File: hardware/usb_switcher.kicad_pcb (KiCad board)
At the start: 2 copper layers, 21 x 52.5 mm, 20 parts, among them U1 MCP1700, U2 IM41_3VDC, U3 IM41_3VDC

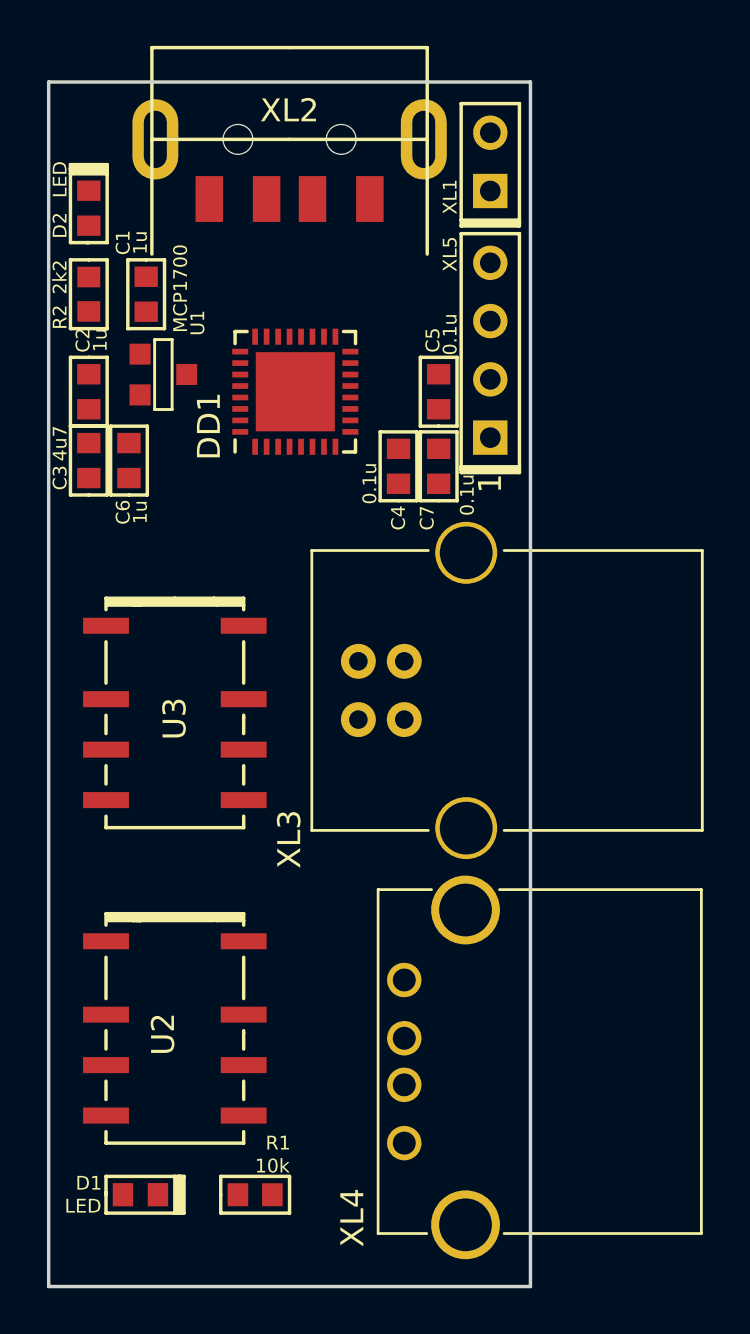
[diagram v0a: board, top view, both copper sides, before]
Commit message: Complete PCB
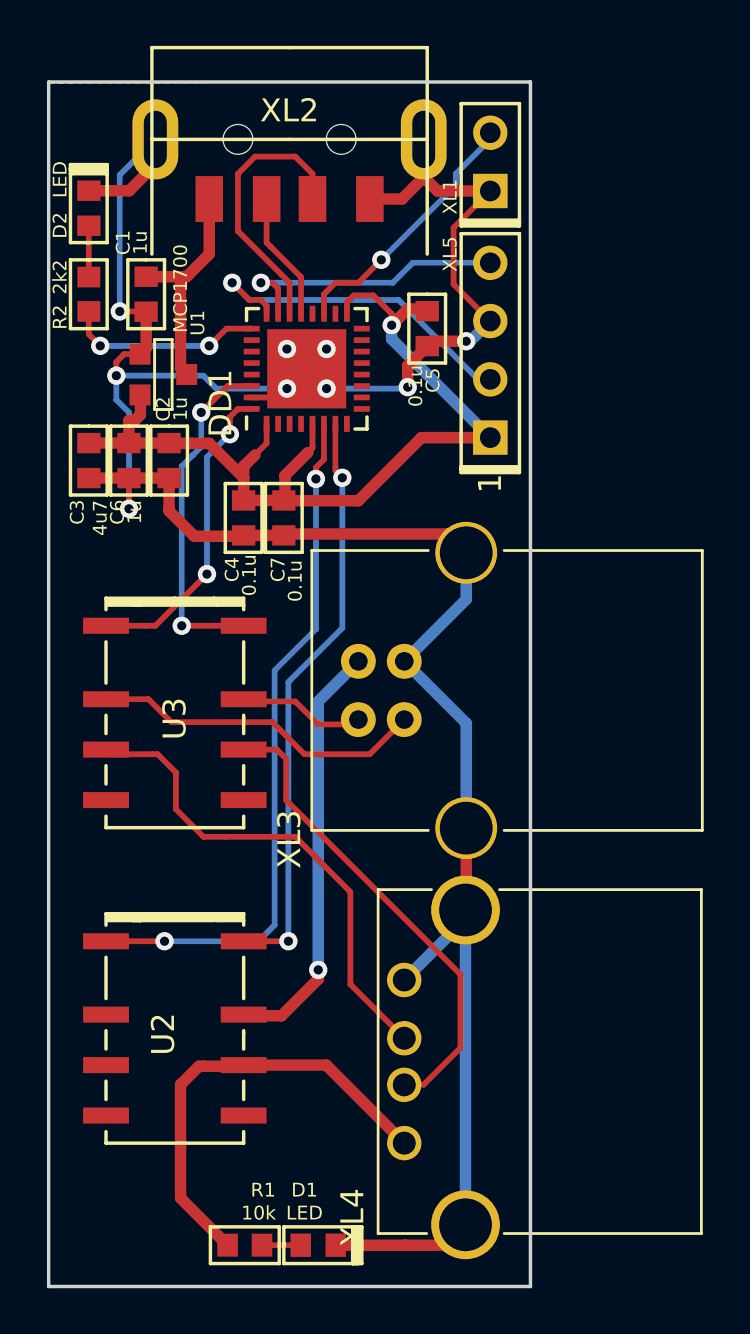
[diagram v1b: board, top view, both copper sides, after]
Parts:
- moved D1 8.06 mm to (181.0, 103.2)
- moved C4 7.12 mm to (177.8, 71.5), turned to 270 degrees
- moved C7 7.12 mm to (179.5, 71.5), turned to 270 degrees
- moved C2 4.61 mm to (174.5, 69.0)
- moved C5 2.80 mm to (185.8, 63.2), turned to 270 degrees
- moved R1 2.25 mm to (177.8, 103.2), turned to 180 degrees
- moved DD1 1.12 mm to (180.5, 65.0)
- turned C3 to 270 degrees
- turned C6 to 270 degrees
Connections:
- DD1 pad 10: /POWER_LED -> Net-(DD1-Pad10)
- DD1 pad 25: Net-(DD1-Pad25) -> /POWER_LED
- DD1 pad 30: Net-(DD1-Pad30) -> /RELAY_DATA_2
- DD1 pad 32: Net-(DD1-Pad32) -> /RELAY_DATA_1
- DD1 pad 8: /RELAY_DATA_1 -> Net-(DD1-Pad8)
- DD1 pad 9: /RELAY_DATA_2 -> Net-(DD1-Pad9)
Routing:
- net GND: track 0.00 -> 125.7 mm, vias 0 -> 9
- net +3.3V: track 0.00 -> 41.6 mm, vias 0 -> 1
- net /RELAY_POWER_1: track 0.00 -> 30.4 mm, vias 0 -> 2
- net /RELAY_POWER_2: track 0.00 -> 25.6 mm, vias 0 -> 2
- net /DEVICE_DP: track 0.00 -> 21.9 mm
- net /DEVICE_DM: track 0.00 -> 20.9 mm
- net /DEVICE_POWER: track 0.00 -> 19.4 mm
- net /HOST_POWER: track 0.00 -> 18.5 mm, vias 0 -> 1
- net /SWCLK: track 0.00 -> 15.3 mm, vias 0 -> 1
- net /RELAY_DATA_2: track 0.00 -> 15.0 mm, vias 0 -> 2
- net /HOST_DP: track 0.00 -> 14.8 mm
- net /RELAY_DATA_1: track 0.00 -> 13.7 mm, vias 0 -> 2
- net /SWDIO: track 0.00 -> 12.3 mm, vias 0 -> 1
- net /USB_DP: track 0.00 -> 12.0 mm
- net /DBG_TX: track 0.00 -> 11.5 mm, vias 0 -> 1
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- added copper zone on B.Cu, net GND
- added copper zone on F.Cu, net GND
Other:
- net class Default: clearance 0.2 -> 0.1; via_dia 0.6 -> 0.8
- net class PWR added: clearance 0.2, trace_width 0.5, via_dia 0.8, via_drill 0.4
- net class Small PWR added: clearance 0.2, trace_width 0.25, via_dia 0.8, via_drill 0.4
- rule trace_clearance: 0.2 -> 0.1

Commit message: + Fix pcd + Add gerber files
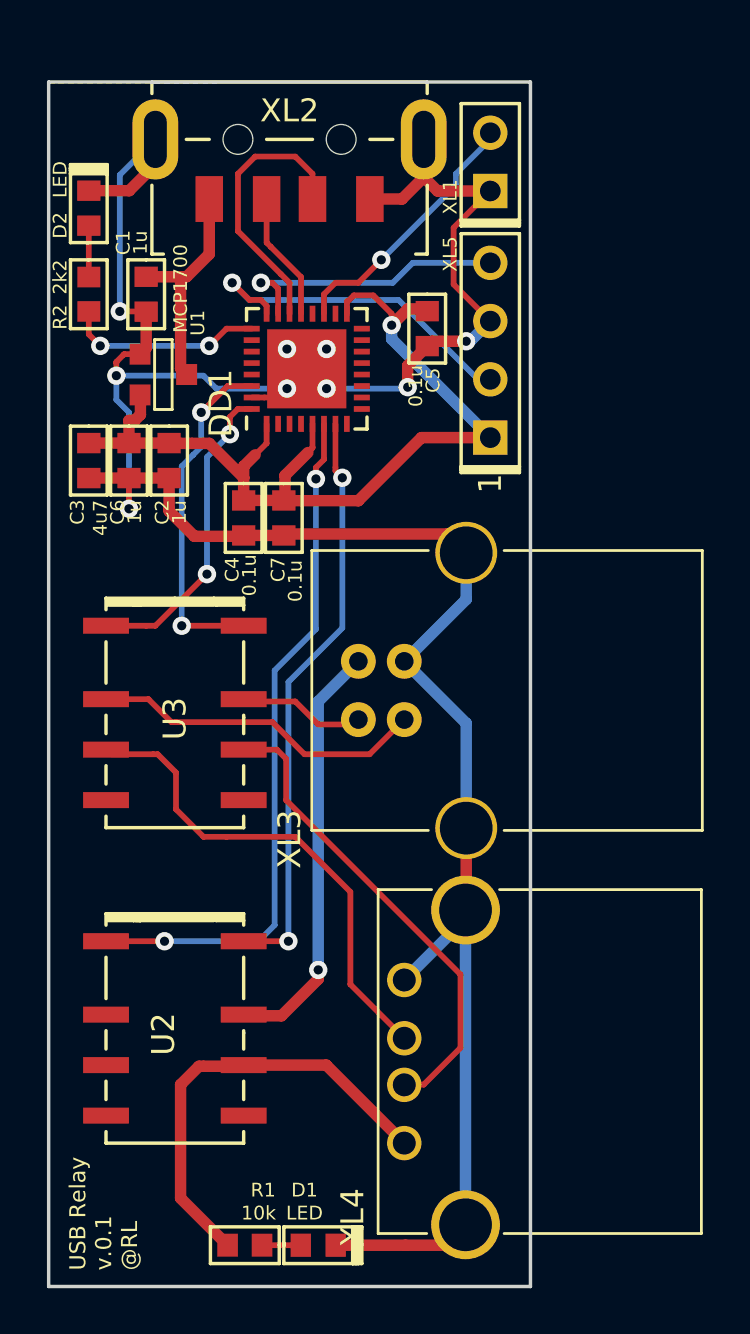
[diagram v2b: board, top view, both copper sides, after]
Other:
- board text added: "USB Relay v.0.1 @RL"
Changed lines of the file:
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@@
     (area 153.000001 47.875 200.725 105.075001)
     (thickness 1.6)
-    (drawings 5)
+    (drawings 6)
     (tracks 265)
     (zones 0)
@@
     (add_net GND)
   )
+  (module Connectors:USB_A_Type2_PCB (layer F.Cu)
+    (at 179.75 55)
+    (descr SHLD)
+    (fp_text reference XL2 (at 0 -1.25) (layer F.SilkS)
+      (effects (font (size 1 1) (thickness 0.15)))
+    )
+    (fp_text value USB_A (at 0 -6) (layer F.Fab)
+      (effects (font (size 1 1) (thickness 0.15)))
+    )
+    (fp_line (start 6 2) (end 6 5) (layer F.SilkS) (width 0.15))
+    (fp_line (start -6 2) (end -6 5) (layer F.SilkS) (width 0.15))
+    (fp_line (start 5.5 5) (end 6 5) (layer F.SilkS) (width 0.15))
+    (fp_line (start -6 5) (end -5.5 5) (layer F.SilkS) (width 0.15))
+    (fp_line (start 3.5 0) (end 4.5 0) (layer F.SilkS) (width 0.15))
+    (fp_line (start -1 0) (end 1 0) (layer F.SilkS) (width 0.15))
+    (fp_line (start -4.5 0) (end -3.5 0) (layer F.SilkS) (width 0.15))
+    (fp_line (start 6 -2.5) (end 6 -2) (layer F.SilkS) (width 0.15))
+    (fp_line (start -6 -2.5) (end -6 -2) (layer F.SilkS) (width 0.15))
+    (fp_line (start -6 -2.5) (end 6 -2.5) (layer F.SilkS) (width 0.15))
+    (pad 1 smd rect (at -3.5 2.6) (size 1.2 2) (layers F.Cu F.Paste F.Mask)
+      (net 1 +5V))
+    (pad 2 smd rect (at -1 2.6) (size 1.2 2) (layers F.Cu F.Paste F.Mask)
+      (net 23 /USB_DM))
+    (pad 3 smd rect (at 1 2.6) (size 1.2 2) (layers F.Cu F.Paste F.Mask)
+      (net 24 /USB_DP))
+    (pad 4 smd rect (at 3.5 2.6) (size 1.2 2) (layers F.Cu F.Paste F.Mask)
+      (net 2 GND))
+    (pad "" np_thru_hole circle (at -2.25 0) (size 1.3 1.3) (drill 1.3) (layers *.Cu *.Mask F.SilkS))
+    (pad "" np_thru_hole circle (at 2.25 0) (size 1.3 1.3) (drill 1.3) (layers *.Cu *.Mask F.SilkS))
+    (pad 5 thru_hole oval (at 5.85 0) (size 2 3.5) (drill oval 1 2.5) (layers *.Cu *.Mask F.SilkS)
+      (net 2 GND))
+    (pad 5 thru_hole oval (at -5.85 0) (size 2 3.5) (drill oval 1 2.5) (layers *.Cu *.Mask F.SilkS)
+      (net 2 GND))
+  )
   (module Capacitors:CAP_0603 (layer F.Cu)
     (at 173.5 61.75 270)
@@
     (at 174.5 69 270)
     (attr smd)
-    (fp_text reference C2 (at -2.25 0.25 450) (layer F.SilkS)
-      (effects (font (size 0.6 0.6) (thickness 0.15)))
-    )
-    (fp_text value 1u (at -2.25 -0.5 270) (layer F.SilkS)
+    (fp_text reference C2 (at 2.25 0.3 450) (layer F.SilkS)
+      (effects (font (size 0.6 0.6) (thickness 0.15)))
+    )
+    (fp_text value 1u (at 2.25 -0.45 270) (layer F.SilkS)
       (effects (font (size 0.6 0.6) (thickness 0.15)))
     )
@@
     )
   )
-  (module Connectors:USB_A_Type2_PCB (layer F.Cu)
-    (at 179.75 55)
-    (descr SHLD)
-    (fp_text reference XL2 (at 0 -1.25) (layer F.SilkS)
-      (effects (font (size 1 1) (thickness 0.15)))
-    )
-    (fp_text value USB_A (at 0 -6) (layer F.Fab)
-      (effects (font (size 1 1) (thickness 0.15)))
-    )
-    (fp_line (start 6 0) (end 6 5) (layer F.SilkS) (width 0.15))
-    (fp_line (start -6 0) (end -6 5) (layer F.SilkS) (width 0.15))
-    (fp_line (start 0 -4) (end 6 -4) (layer F.SilkS) (width 0.15))
-    (fp_line (start 6 -4) (end 6 0) (layer F.SilkS) (width 0.15))
-    (fp_line (start 0 -4) (end -6 -4) (layer F.SilkS) (width 0.15))
-    (fp_line (start -6 -4) (end -6 0) (layer F.SilkS) (width 0.15))
-    (fp_line (start 0 0) (end 6 0) (layer F.SilkS) (width 0.15))
-    (fp_line (start 0 0) (end -6 0) (layer F.SilkS) (width 0.15))
-    (pad 1 smd rect (at -3.5 2.6) (size 1.2 2) (layers F.Cu F.Paste F.Mask)
-      (net 1 +5V))
-    (pad 2 smd rect (at -1 2.6) (size 1.2 2) (layers F.Cu F.Paste F.Mask)
-      (net 23 /USB_DM))
-    (pad 3 smd rect (at 1 2.6) (size 1.2 2) (layers F.Cu F.Paste F.Mask)
-      (net 24 /USB_DP))
-    (pad 4 smd rect (at 3.5 2.6) (size 1.2 2) (layers F.Cu F.Paste F.Mask)
-      (net 2 GND))
-    (pad "" np_thru_hole circle (at -2.25 0) (size 1.3 1.3) (drill 1.3) (layers *.Cu *.Mask F.SilkS))
-    (pad "" np_thru_hole circle (at 2.25 0) (size 1.3 1.3) (drill 1.3) (layers *.Cu *.Mask F.SilkS))
-    (pad 5 thru_hole oval (at 5.85 0) (size 2 3.5) (drill oval 1 2.5) (layers *.Cu *.Mask F.SilkS)
-      (net 2 GND))
-    (pad 5 thru_hole oval (at -5.85 0) (size 2 3.5) (drill oval 1 2.5) (layers *.Cu *.Mask F.SilkS)
-      (net 2 GND))
-  )
   (module Connectors:PLS-4 (layer F.Cu)
     (at 188.5 68 90)
@@
       (net 41 /SWDIO))
   )
+  (gr_text "USB Relay\nv.0.1\n@RL" (at 171.65 104.3 90) (layer F.SilkS)
+    (effects (font (size 0.7 0.7) (thickness 0.175)) (justify left))
+  )
   (gr_line (start 169.25 105) (end 169.25 52.5) (angle 90) (layer Edge.Cuts) (width 0.15))
   (gr_line (start 190.25 105) (end 169.25 105) (angle 90) (layer Edge.Cuts) (width 0.15))
@@
   (segment (start 172.2 66.35) (end 172.75 66.9) (width 0.25) (layer B.Cu) (net 2))
   (segment (start 172.2 65.3) (end 172.2 66.35) (width 0.25) (layer B.Cu) (net 2))
-  (segment (start 172.75 71.1) (end 172.75 69.762) (width 0.25) (layer F.Cu) (net 2) (status 800000))
+  (segment (start 172.75 71.1) (end 172.75 69.762) (width 0.25) (layer F.Cu) (net 2))
   (via (at 172.75 71.1) (size 0.8) (drill 0.4) (layers F.Cu B.Cu) (net 2))
   (segment (start 172.75 66.9) (end 172.75 71.1) (width 0.25) (layer B.Cu) (net 2))
